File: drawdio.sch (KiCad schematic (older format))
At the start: 23 parts, among them P1 CONN_01X01, P10 CONN_01X02, P2 CONN_01X01, P3 CONN_01X01, P4 CONN_01X02, P5 CONN_01X01, P6 CONN_01X01, P7 CONN_01X01, P9 CONN_02X04, Q1 BC558, Q2 BC547, Q3 BC558, Q4 BC547, U1 LM555N

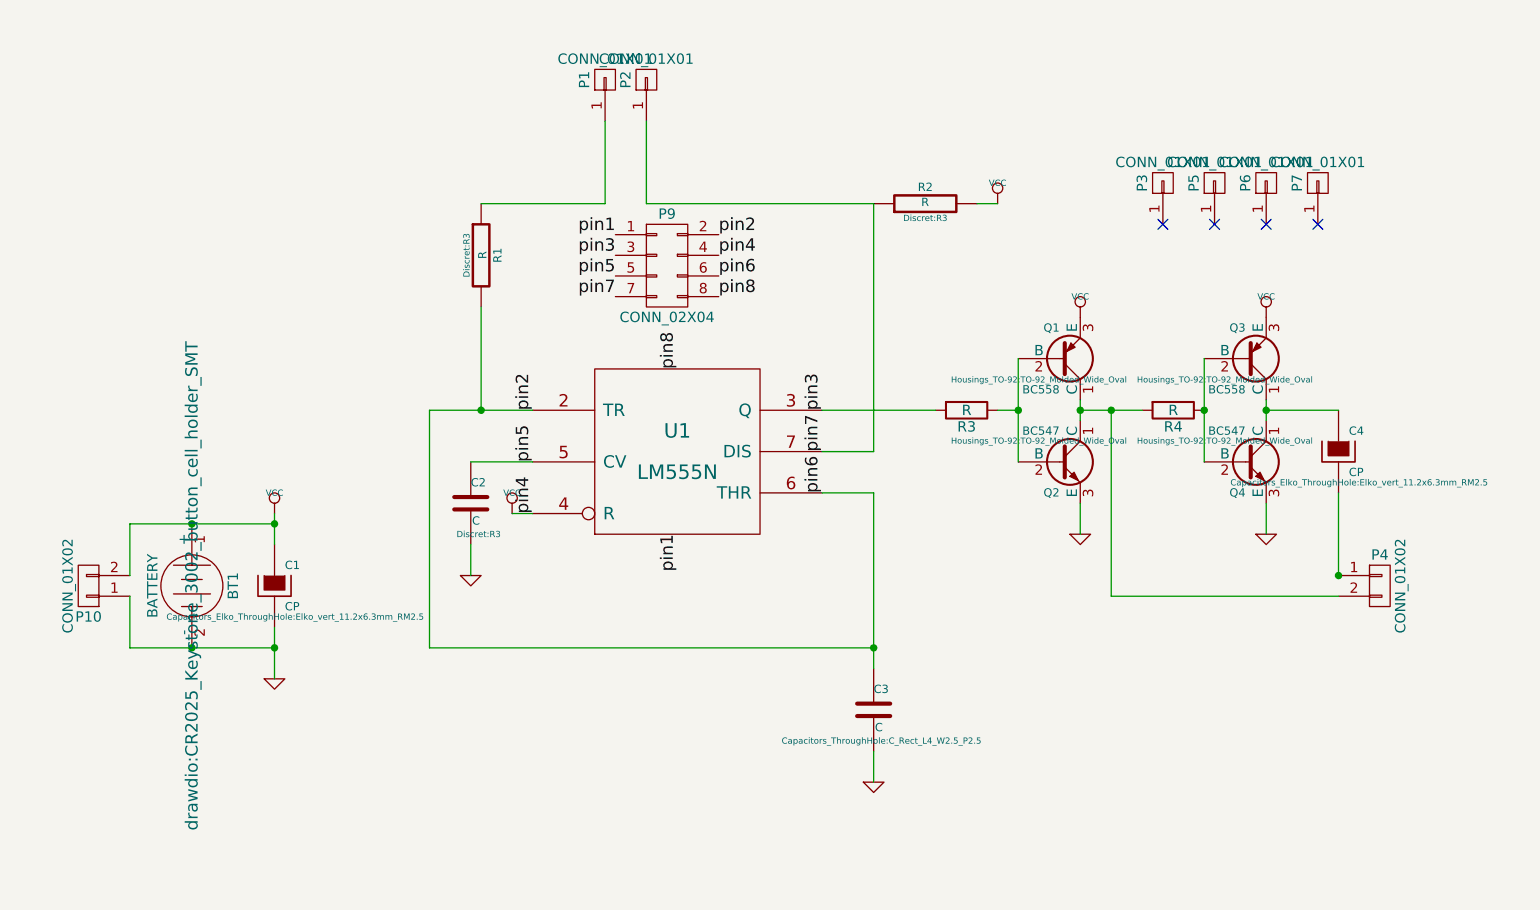
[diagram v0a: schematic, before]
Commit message: Wiki is coming
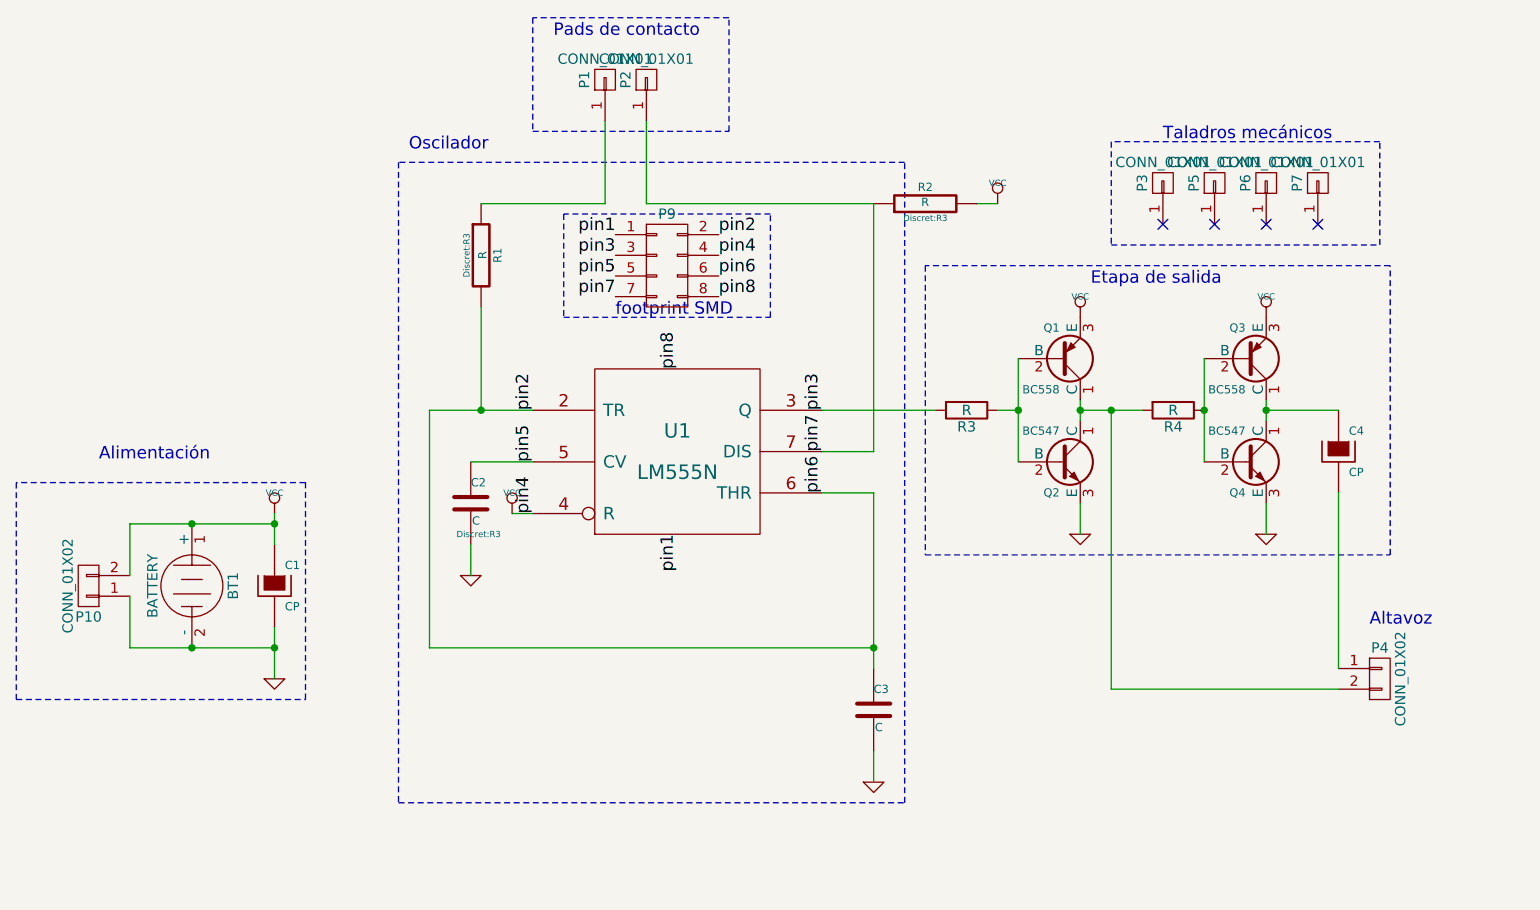
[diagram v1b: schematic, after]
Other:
- note added: "Alimentación"
- note added: "Altavoz"
- note added: "Etapa de salida"
- note added: "Oscilador"
- note added: "Pads de contacto"
- note added: "Taladros mecánicos"
- note added: "footprint SMD"
- moved on the sheet: P4
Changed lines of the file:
@@
 LIBS:memory
 LIBS:xilinx
-LIBS:special
 LIBS:microcontrollers
 LIBS:dsp
@@
 encoding utf-8
 Sheet 1 1
-Title ""
+Title "Drawdio"
 Date "20 apr 2015"
-Rev ""
-Comp ""
-Comment1 ""
-Comment2 ""
+Rev "V1.0"
+Comp "UC3Music"
+Comment1 "Originally designed by Jay Silver"
+Comment2 "Upgrades on output stage by JorFru"
 Comment3 ""
 Comment4 ""
@@
 F 0 "Q3" H 8350 3351 40  0000 R CNN
 F 1 "BC558" H 8350 3650 40  0000 R CNN
-F 2 "Housings_TO-92:TO-92_Molded_Wide_Oval" H 8250 3602 29  0000 C CNN
+F 2 "Housings_TO-92:TO-92_Molded_Wide_Oval" H 7700 3600 29  0001 C CNN
 F 3 "" H 8350 3500 60  0000 C CNN
 	1    8350 3500
@@
 F 0 "C4" H 8850 4050 40  0000 L CNN
 F 1 "CP" H 8850 3850 40  0000 L CNN
-F 2 "Capacitors_Elko_ThroughHole:Elko_vert_11.2x6.3mm_RM2.5" H 8900 3800 30  0000 C CNN
+F 2 "Capacitors_Elko_ThroughHole:Elko_vert_11.2x6.3mm_RM2.5" H 8900 3800 30  0001 C CNN
 F 3 "~" H 8800 3950 300 0000 C CNN
 	1    8800 3950
@@
 F 0 "C3" H 6550 5300 40  0000 L CNN
 F 1 "C" H 6556 5115 40  0000 L CNN
-F 2 "Capacitors_ThroughHole:C_Rect_L4_W2.5_P2.5" H 6588 5050 30  0000 C CNN
+F 2 "Capacitors_ThroughHole:C_Rect_L4_W2.5_P2.5" H 6588 5050 30  0001 C CNN
 F 3 "~" H 6550 5200 60  0000 C CNN
 	1    6550 5200
@@
 F 0 "C1" H 3700 4700 40  0000 L CNN
 F 1 "CP" H 3700 4500 40  0000 L CNN
-F 2 "Capacitors_Elko_ThroughHole:Elko_vert_11.2x6.3mm_RM2.5" H 3750 4450 30  0000 C CNN
+F 2 "Capacitors_Elko_ThroughHole:Elko_vert_11.2x6.3mm_RM2.5" H 7850 5600 30  0001 C CNN
 F 3 "~" H 3650 4600 300 0000 C CNN
 	1    3650 4600
@@
 F 0 "BT1" H 3250 4800 50  0000 C CNN
 F 1 "BATTERY" H 3250 4410 50  0000 C CNN
-F 2 "drawdio:CR2025_Keystone_3002_button_cell_holder_SMT" H 3250 4600 60  0000 C CNN
+F 2 "drawdio:CR2025_Keystone_3002_button_cell_holder_SMT" H 3400 5350 60  0001 C CNN
 F 3 "~" H 3250 4600 60  0000 C CNN
 	1    3250 4600
@@
 F 0 "Q4" H 8350 3851 40  0000 R CNN
 F 1 "BC547" H 8350 4150 40  0000 R CNN
-F 2 "Housings_TO-92:TO-92_Molded_Wide_Oval" H 8250 4102 29  0000 C CNN
+F 2 "Housings_TO-92:TO-92_Molded_Wide_Oval" H 8250 4102 29  0001 C CNN
 F 3 "" H 8350 4000 60  0000 C CNN
 	1    8350 4000
@@
 F 0 "Q1" H 7450 3351 40  0000 R CNN
 F 1 "BC558" H 7450 3650 40  0000 R CNN
-F 2 "Housings_TO-92:TO-92_Molded_Wide_Oval" H 7350 3602 29  0000 C CNN
+F 2 "Housings_TO-92:TO-92_Molded_Wide_Oval" H 7350 3602 29  0001 C CNN
 F 3 "" H 7450 3500 60  0000 C CNN
 	1    7450 3500
@@
 F 0 "Q2" H 7450 3851 40  0000 R CNN
 F 1 "BC547" H 7450 4150 40  0000 R CNN
-F 2 "Housings_TO-92:TO-92_Molded_Wide_Oval" H 7350 4102 29  0000 C CNN
+F 2 "Housings_TO-92:TO-92_Molded_Wide_Oval" V 7350 4102 29  0001 C CNN
 F 3 "" H 7450 4000 60  0000 C CNN
 	1    7450 4000
@@
 L CONN_01X02 P4
 U 1 1 562400DE
-P 9000 4600
-F 0 "P4" H 9000 4750 50  0000 C CNN
-F 1 "CONN_01X02" V 9100 4600 50  0000 C CNN
-F 2 "drawdio:RS_mini_speaker_724-3100" H 9000 4600 60  0001 C CNN
-F 3 "" H 9000 4600 60  0000 C CNN
-	1    9000 4600
+P 9000 5050
+F 0 "P4" H 9000 5200 50  0000 C CNN
+F 1 "CONN_01X02" V 9100 5050 50  0000 C CNN
+F 2 "drawdio:RS_mini_speaker_724-3100" H 9000 5050 60  0001 C CNN
+F 3 "" H 9000 5050 60  0000 C CNN
+	1    9000 5050
 	1    0    0    -1
 $EndComp
@@
 Wire Wire Line
 	4600 4550 4600 4400
-Connection ~ 8800 4550
 Wire Wire Line
 	7550 4350 7550 4200
@@
 Connection ~ 8150 3750
 Wire Wire Line
-	8800 4150 8800 4550
+	8800 4150 8800 5000
 Wire Wire Line
 	8450 3700 8450 3800
 Connection ~ 8450 3750
 Wire Wire Line
-	7700 3750 7700 4650
-Wire Wire Line
-	7700 4650 8800 4650
+	7700 3750 7700 5100
+Wire Wire Line
+	7700 5100 8800 5100
 Connection ~ 7700 3750
 $Comp
@@
 P 5550 3050
 F 0 "P9" H 5550 3300 50  0000 C CNN
-F 1 "CONN_02X04" H 5550 2800 50  0000 C CNN
+F 1 "CONN_02X04" H 5550 2800 50  0001 C CNN
 F 2 "Housings_SOIC:SOIC-8_3.9x4.9mm_Pitch1.27mm" H 5550 1850 60  0001 C CNN
 F 3 "" H 5550 1850 60  0000 C CNN
@@
 	2950 4650 2950 4900
 Connection ~ 3250 4900
+Wire Notes Line
+	6800 3050 6800 4450
+Wire Notes Line
+	6800 4450 9050 4450
+Wire Notes Line
+	9050 4450 9050 3050
+Wire Notes Line
+	9050 3050 6800 3050
+Wire Notes Line
+	7700 2450 7700 2950
+Wire Notes Line
+	7700 2950 9000 2950
+Wire Notes Line
+	9000 2950 9000 2450
+Wire Notes Line
+	9000 2450 7700 2450
+Text Notes 8950 4800 0    60   ~ 0
+Altavoz
+Text Notes 7600 3150 0    60   ~ 0
+Etapa de salida
+Text Notes 7950 2450 0    60   ~ 0
+Taladros mecánicos
+Wire Notes Line
+	2400 4100 2400 5150
+Wire Notes Line
+	2400 5150 3800 5150
+Wire Notes Line
+	3800 5150 3800 4100
+Wire Notes Line
+	3800 4100 2400 4100
+Text Notes 2800 4000 0    60   ~ 0
+Alimentación
+Wire Notes Line
+	4900 1850 4900 2400
+Wire Notes Line
+	4900 2400 5850 2400
+Wire Notes Line
+	5850 2400 5850 1850
+Wire Notes Line
+	5850 1850 4900 1850
+Text Notes 5000 1950 0    60   ~ 0
+Pads de contacto
+Wire Notes Line
+	4250 2550 4250 5650
+Wire Notes Line
+	4250 5650 6700 5650
+Wire Notes Line
+	6700 5650 6700 2550
+Wire Notes Line
+	6700 2550 4250 2550
+Text Notes 4300 2500 0    60   ~ 0
+Oscilador
+Wire Notes Line
+	5050 2800 5050 3300
+Wire Notes Line
+	5050 3300 6050 3300
+Wire Notes Line
+	6050 3300 6050 2800
+Wire Notes Line
+	6050 2800 5050 2800
+Text Notes 5300 3300 0    60   ~ 0
+footprint SMD
 $EndSCHEMATC
